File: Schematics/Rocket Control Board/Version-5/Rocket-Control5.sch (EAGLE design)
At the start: 29 parts

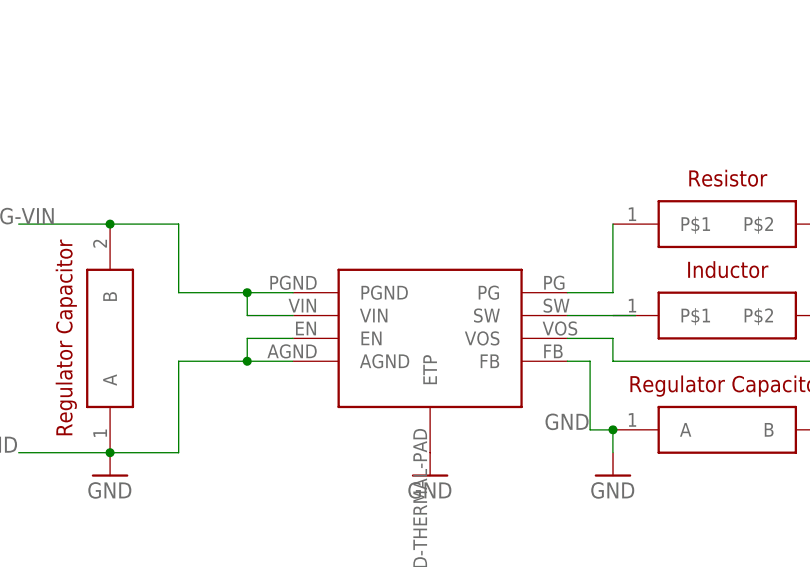
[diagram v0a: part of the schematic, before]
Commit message: Final commit for the semester
Various board changes.
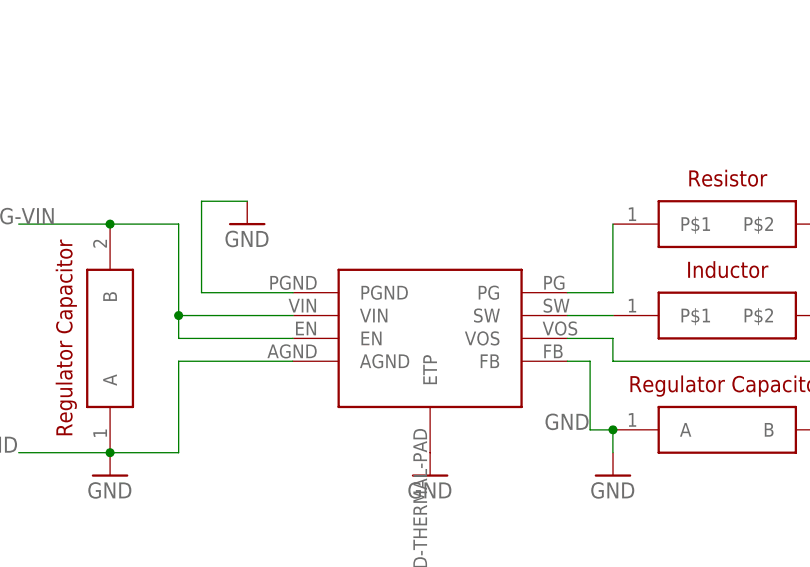
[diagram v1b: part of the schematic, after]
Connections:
- net GND: now also U$5.PGND; no longer U$5.EN
- net REG-VIN: now also U$5.EN; no longer U$5.PGND
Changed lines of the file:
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@@
 <part name="U$20" library="RocketControlBoard" deviceset="I2C-PULLUP" device=""/>
 <part name="+3V10" library="supply1" deviceset="+3V3" device=""/>
+<part name="GND19" library="supply1" deviceset="GND" device=""/>
 </parts>
 <sheets>
@@
 <instance part="U$20" gate="G$1" x="157.48" y="-99.06"/>
 <instance part="+3V10" gate="G$1" x="177.8" y="-81.28"/>
+<instance part="GND19" gate="1" x="-81.28" y="-35.56"/>
 </instances>
 <busses>
@@
 </segment>
 <segment>
-<pinref part="U$5" gate="G$1" pin="AGND"/>
-<wire x1="-76.2" y1="-50.8" x2="-81.28" y2="-50.8" width="0.1524" layer="91"/>
-<wire x1="-81.28" y1="-50.8" x2="-88.9" y2="-50.8" width="0.1524" layer="91"/>
 <wire x1="-88.9" y1="-50.8" x2="-88.9" y2="-60.96" width="0.1524" layer="91"/>
 <pinref part="U$11" gate="G$1" pin="A"/>
 <wire x1="-88.9" y1="-60.96" x2="-96.52" y2="-60.96" width="0.1524" layer="91"/>
-<pinref part="U$5" gate="G$1" pin="EN"/>
-<wire x1="-76.2" y1="-48.26" x2="-81.28" y2="-48.26" width="0.1524" layer="91"/>
-<wire x1="-81.28" y1="-48.26" x2="-81.28" y2="-50.8" width="0.1524" layer="91"/>
 <wire x1="-96.52" y1="-60.96" x2="-106.68" y2="-60.96" width="0.1524" layer="91"/>
 <pinref part="GND10" gate="1" pin="GND"/>
 <junction x="-96.52" y="-60.96"/>
 <label x="-111.76" y="-60.96" size="1.778" layer="95"/>
-<junction x="-81.28" y="-50.8"/>
+<pinref part="U$5" gate="G$1" pin="AGND"/>
+<wire x1="-76.2" y1="-50.8" x2="-88.9" y2="-50.8" width="0.1524" layer="91"/>
 </segment>
 <segment>
@@
 <wire x1="15.24" y1="-91.44" x2="22.86" y2="-91.44" width="0.1524" layer="91"/>
 <wire x1="22.86" y1="-91.44" x2="22.86" y2="-93.98" width="0.1524" layer="91"/>
+</segment>
+<segment>
+<pinref part="GND19" gate="1" pin="GND"/>
+<wire x1="-81.28" y1="-33.02" x2="-86.36" y2="-33.02" width="0.1524" layer="91"/>
+<wire x1="-86.36" y1="-33.02" x2="-86.36" y2="-43.18" width="0.1524" layer="91"/>
+<pinref part="U$5" gate="G$1" pin="PGND"/>
+<wire x1="-76.2" y1="-43.18" x2="-86.36" y2="-43.18" width="0.1524" layer="91"/>
 </segment>
 </net>
@@
 <pinref part="U$13" gate="G$1" pin="P$1"/>
 <wire x1="-45.72" y1="-45.72" x2="-40.64" y2="-45.72" width="0.1524" layer="91"/>
-<wire x1="-38.1" y1="-45.72" x2="-40.64" y2="-45.72" width="0.1524" layer="91"/>
 </segment>
 </net>
 <net name="REG-VIN" class="0">
 <segment>
-<pinref part="U$5" gate="G$1" pin="PGND"/>
-<wire x1="-76.2" y1="-43.18" x2="-81.28" y2="-43.18" width="0.1524" layer="91"/>
-<wire x1="-81.28" y1="-43.18" x2="-88.9" y2="-43.18" width="0.1524" layer="91"/>
-<wire x1="-88.9" y1="-43.18" x2="-88.9" y2="-35.56" width="0.1524" layer="91"/>
+<wire x1="-88.9" y1="-45.72" x2="-88.9" y2="-35.56" width="0.1524" layer="91"/>
 <pinref part="U$11" gate="G$1" pin="B"/>
 <wire x1="-88.9" y1="-35.56" x2="-96.52" y2="-35.56" width="0.1524" layer="91"/>
-<pinref part="U$5" gate="G$1" pin="VIN"/>
-<wire x1="-76.2" y1="-45.72" x2="-81.28" y2="-45.72" width="0.1524" layer="91"/>
-<wire x1="-81.28" y1="-45.72" x2="-81.28" y2="-43.18" width="0.1524" layer="91"/>
 <wire x1="-96.52" y1="-35.56" x2="-106.68" y2="-35.56" width="0.1524" layer="91"/>
 <label x="-111.76" y="-35.56" size="1.778" layer="95"/>
-<junction x="-81.28" y="-43.18"/>
 <junction x="-96.52" y="-35.56"/>
-</segment>
-<segment>
+<pinref part="U$5" gate="G$1" pin="VIN"/>
+<wire x1="-76.2" y1="-45.72" x2="-88.9" y2="-45.72" width="0.1524" layer="91"/>
+<pinref part="U$5" gate="G$1" pin="EN"/>
+<wire x1="-76.2" y1="-48.26" x2="-88.9" y2="-48.26" width="0.1524" layer="91"/>
+<wire x1="-88.9" y1="-48.26" x2="-88.9" y2="-45.72" width="0.1524" layer="91"/>
+<junction x="-88.9" y="-45.72"/>
+</segment>
+<segment>
